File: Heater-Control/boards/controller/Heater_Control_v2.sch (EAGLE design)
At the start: 4 parts, among them J1 S2B-XH-A(LF)(SN), U1 QT Py #4600, X1 MLX-43860

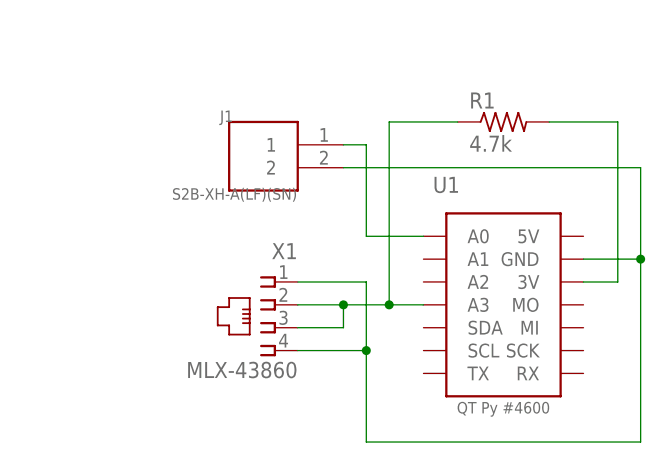
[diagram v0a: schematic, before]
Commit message: updated control board
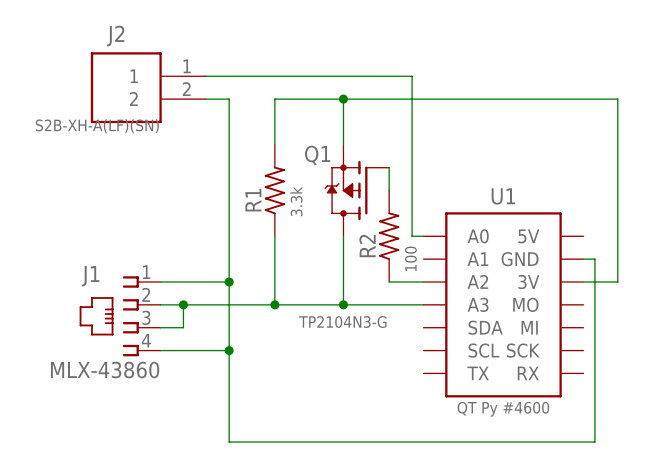
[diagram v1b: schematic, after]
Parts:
- removed X1: MLX-43860, home:MLX-43860
- added J2: S2B-XH-A(LF)(SN), Connectors:S2B-XH-A(LF)(SN)
- added Q1: TP2104N3-G, home:MOSFET-PCH-TO92
- added R2: 100, home:R-US_R1206
- J1: value S2B-XH-A(LF)(SN) -> MLX-43860; device Connectors:S2B-XH-A(LF)(SN) -> home:MLX-43860
- R1: value 4.7k -> 3.3k
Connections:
- new net GATE: Q1.G, R2.2
- new net SPU_GATE: R2.1, U1.A2
- net 3V3: now also Q1.S
- net DATA-1WIRE: now also J1.2, J1.3, Q1.D; no longer X1.2, X1.3
- net GND: now also J1.1, J1.4, J2.2; no longer J1.2, X1.1, X1.4
- net PWR: now also J2.1; no longer J1.1
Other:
- moved on the sheet: R1
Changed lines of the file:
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@@
 <setting verticaltext="up"/>
 </settings>
-<grid distance="0.1" unitdist="inch" unit="inch" style="lines" multiple="1" display="yes" altdistance="0.01" altunitdist="inch" altunit="inch"/>
+<grid distance="100" unitdist="mil" unit="mil" style="lines" multiple="1" display="yes" altdistance="50" altunitdist="mil" altunit="mil"/>
 <layers>
 <layer number="1" name="Top" color="4" fill="1" visible="no" active="no"/>
@@
 <class number="1" name="10mil" width="0.254" drill="0">
 </class>
+<class number="2" name="12mil" width="0.3048" drill="0">
+</class>
+<class number="3" name="8mil" width="0.2032" drill="0">
+</class>
 </classes>
 <parts>
 <part name="U1" library="home" deviceset="QT_PY" device="" value="QT Py #4600"/>
-<part name="X1" library="home" deviceset="MLX-43860" device=""/>
-<part name="J1" library="Connectors" library_urn="urn:adsk.eagle:library:14555660" deviceset="S2B-XH-A(LF)(SN)" device="" package3d_urn="urn:adsk.eagle:package:10989915/2"/>
-<part name="R1" library="home" deviceset="R-US_" device="R1206" package3d_urn="urn:adsk.eagle:package:23540/2" value="4.7k"/>
+<part name="J1" library="home" deviceset="MLX-43860" device=""/>
+<part name="J2" library="Connectors" library_urn="urn:adsk.eagle:library:14555660" deviceset="S2B-XH-A(LF)(SN)" device="" package3d_urn="urn:adsk.eagle:package:10989915/2"/>
+<part name="R1" library="home" deviceset="R-US_" device="R1206" package3d_urn="urn:adsk.eagle:package:23540/2" value="3.3k"/>
+<part name="Q1" library="home" deviceset="MOSFET-PCH" device="-TO92" value="TP2104N3-G"/>
+<part name="R2" library="home" deviceset="R-US_" device="R1206" package3d_urn="urn:adsk.eagle:package:23540/2" value="100"/>
 </parts>
 <sheets>
@@
 <instances>
 <instance part="U1" gate="G$1" x="38.1" y="15.24" smashed="yes">
-<attribute name="NAME" x="31.75" y="27.686" size="1.778" layer="95" ratio="10" align="bottom-center"/>
+<attribute name="NAME" x="38.1" y="26.416" size="1.778" layer="95" ratio="10" align="bottom-center"/>
 <attribute name="VALUE" x="38.1" y="4.445" size="1.27" layer="96" ratio="10" rot="R180" align="bottom-center"/>
 </instance>
-<instance part="X1" gate="G$1" x="12.7" y="12.7" smashed="yes" rot="MR0">
-<attribute name="NAME" x="15.24" y="20.32" size="1.778" layer="95" rot="MR0"/>
-<attribute name="VALUE" x="15.24" y="7.112" size="1.778" layer="96" rot="MR0"/>
-</instance>
-<instance part="J1" gate="G$1" x="10.16" y="30.48" smashed="yes">
-<attribute name="NAME" x="6.604" y="35.56" size="1.27" layer="95"/>
-<attribute name="VALUE" x="1.27" y="26.924" size="1.27" layer="96"/>
-</instance>
-<instance part="R1" gate="G$1" x="38.1" y="35.56" smashed="yes">
-<attribute name="NAME" x="34.29" y="37.0586" size="1.778" layer="95"/>
-<attribute name="VALUE" x="34.29" y="32.258" size="1.778" layer="96"/>
+<instance part="J1" gate="G$1" x="-2.54" y="12.7" smashed="yes" rot="MR0">
+<attribute name="NAME" x="-7.62" y="17.78" size="1.778" layer="95" ratio="10" rot="MR0" align="bottom-center"/>
+<attribute name="VALUE" x="0" y="7.112" size="1.778" layer="96" rot="MR0"/>
+</instance>
+<instance part="J2" gate="G$1" x="-5.08" y="38.1" smashed="yes">
+<attribute name="NAME" x="-4.826" y="44.45" size="1.778" layer="95" ratio="10" align="bottom-center"/>
+<attribute name="VALUE" x="-13.97" y="34.544" size="1.27" layer="96"/>
+</instance>
+<instance part="R1" gate="G$1" x="12.7" y="27.94" smashed="yes" rot="R90">
+<attribute name="NAME" x="11.2014" y="25.4" size="1.778" layer="95" ratio="10" rot="R90"/>
+<attribute name="VALUE" x="14.478" y="26.67" size="1.27" layer="96" ratio="10" rot="R270" align="bottom-center"/>
+</instance>
+<instance part="Q1" gate="G$1" x="20.32" y="27.94" smashed="yes" rot="MR0">
+<attribute name="VALUE" x="20.32" y="13.97" size="1.27" layer="96" rot="MR180" align="bottom-center"/>
+<attribute name="NAME" x="19.05" y="31.115" size="1.778" layer="95" ratio="10" rot="MR0"/>
+</instance>
+<instance part="R2" gate="G$1" x="25.4" y="22.86" smashed="yes" rot="R90">
+<attribute name="NAME" x="23.9014" y="20.32" size="1.778" layer="95" ratio="10" rot="R90"/>
+<attribute name="VALUE" x="27.178" y="20.32" size="1.27" layer="96" ratio="10" rot="R270" align="bottom-center"/>
 </instance>
 </instances>
@@
 </busses>
 <nets>
-<net name="GND" class="1">
+<net name="GND" class="2">
 <segment>
 <pinref part="U1" gate="G$1" pin="GND"/>
-<pinref part="X1" gate="G$1" pin="4"/>
-<wire x1="46.99" y1="20.32" x2="53.34" y2="20.32" width="0.1524" layer="91"/>
-<wire x1="15.24" y1="10.16" x2="22.86" y2="10.16" width="0.1524" layer="91"/>
-<wire x1="22.86" y1="10.16" x2="22.86" y2="0" width="0.1524" layer="91"/>
-<wire x1="22.86" y1="0" x2="53.34" y2="0" width="0.1524" layer="91"/>
-<wire x1="53.34" y1="0" x2="53.34" y2="20.32" width="0.1524" layer="91"/>
-<junction x="53.34" y="20.32"/>
-<pinref part="X1" gate="G$1" pin="1"/>
-<wire x1="15.24" y1="17.78" x2="22.86" y2="17.78" width="0.1524" layer="91"/>
-<wire x1="22.86" y1="17.78" x2="22.86" y2="10.16" width="0.1524" layer="91"/>
-<junction x="22.86" y="10.16"/>
-<wire x1="53.34" y1="30.48" x2="53.34" y2="20.32" width="0.1524" layer="91"/>
-<pinref part="J1" gate="G$1" pin="2"/>
-<wire x1="20.32" y1="30.48" x2="53.34" y2="30.48" width="0.1524" layer="91"/>
-</segment>
-</net>
-<net name="3V3" class="1">
+<pinref part="J1" gate="G$1" pin="4"/>
+<wire x1="46.99" y1="20.32" x2="48.26" y2="20.32" width="0.1524" layer="91"/>
+<wire x1="0" y1="10.16" x2="7.62" y2="10.16" width="0.1524" layer="91"/>
+<wire x1="7.62" y1="10.16" x2="7.62" y2="0" width="0.1524" layer="91"/>
+<wire x1="7.62" y1="0" x2="48.26" y2="0" width="0.1524" layer="91"/>
+<wire x1="48.26" y1="0" x2="48.26" y2="20.32" width="0.1524" layer="91"/>
+<pinref part="J1" gate="G$1" pin="1"/>
+<wire x1="0" y1="17.78" x2="7.62" y2="17.78" width="0.1524" layer="91"/>
+<wire x1="7.62" y1="17.78" x2="7.62" y2="10.16" width="0.1524" layer="91"/>
+<junction x="7.62" y="10.16"/>
+<pinref part="J2" gate="G$1" pin="2"/>
+<wire x1="5.08" y1="38.1" x2="7.62" y2="38.1" width="0.1524" layer="91"/>
+<wire x1="7.62" y1="17.78" x2="7.62" y2="38.1" width="0.1524" layer="91"/>
+<junction x="7.62" y="17.78"/>
+</segment>
+</net>
+<net name="3V3" class="2">
 <segment>
 <pinref part="U1" gate="G$1" pin="3V"/>
 <wire x1="46.99" y1="17.78" x2="50.8" y2="17.78" width="0.1524" layer="91"/>
 <pinref part="R1" gate="G$1" pin="2"/>
-<wire x1="50.8" y1="17.78" x2="50.8" y2="35.56" width="0.1524" layer="91"/>
-<wire x1="50.8" y1="35.56" x2="43.18" y2="35.56" width="0.1524" layer="91"/>
-</segment>
-</net>
-<net name="DATA-1WIRE" class="1">
-<segment>
-<pinref part="X1" gate="G$1" pin="2"/>
-<pinref part="X1" gate="G$1" pin="3"/>
-<wire x1="20.32" y1="15.24" x2="15.24" y2="15.24" width="0.1524" layer="91"/>
-<wire x1="15.24" y1="12.7" x2="20.32" y2="12.7" width="0.1524" layer="91"/>
-<wire x1="20.32" y1="12.7" x2="20.32" y2="15.24" width="0.1524" layer="91"/>
+<wire x1="50.8" y1="17.78" x2="50.8" y2="38.1" width="0.1524" layer="91"/>
+<wire x1="50.8" y1="38.1" x2="20.32" y2="38.1" width="0.1524" layer="91"/>
+<wire x1="12.7" y1="38.1" x2="12.7" y2="33.02" width="0.1524" layer="91"/>
+<wire x1="12.7" y1="38.1" x2="20.32" y2="38.1" width="0.1524" layer="91"/>
+<pinref part="Q1" gate="G$1" pin="S"/>
+<wire x1="20.32" y1="38.1" x2="20.32" y2="33.02" width="0.1524" layer="91"/>
+<junction x="20.32" y="38.1"/>
+</segment>
+</net>
+<net name="DATA-1WIRE" class="2">
+<segment>
+<pinref part="J1" gate="G$1" pin="2"/>
+<pinref part="J1" gate="G$1" pin="3"/>
+<wire x1="2.54" y1="15.24" x2="0" y2="15.24" width="0.1524" layer="91"/>
+<wire x1="0" y1="12.7" x2="2.54" y2="12.7" width="0.1524" layer="91"/>
+<wire x1="2.54" y1="12.7" x2="2.54" y2="15.24" width="0.1524" layer="91"/>
 <pinref part="U1" gate="G$1" pin="A3"/>
-<wire x1="29.21" y1="15.24" x2="25.4" y2="15.24" width="0.1524" layer="91"/>
+<wire x1="29.21" y1="15.24" x2="20.32" y2="15.24" width="0.1524" layer="91"/>
+<pinref part="R1" gate="G$1" pin="1"/>
+<wire x1="20.32" y1="15.24" x2="12.7" y2="15.24" width="0.1524" layer="91"/>
+<wire x1="12.7" y1="22.86" x2="12.7" y2="15.24" width="0.1524" layer="91"/>
+<junction x="12.7" y="15.24"/>
+<wire x1="2.54" y1="15.24" x2="12.7" y2="15.24" width="0.1524" layer="91"/>
+<junction x="2.54" y="15.24"/>
+<pinref part="Q1" gate="G$1" pin="D"/>
+<wire x1="20.32" y1="22.86" x2="20.32" y2="15.24" width="0.1524" layer="91"/>
 <junction x="20.32" y="15.24"/>
-<pinref part="R1" gate="G$1" pin="1"/>
-<wire x1="25.4" y1="15.24" x2="20.32" y2="15.24" width="0.1524" layer="91"/>
-<wire x1="33.02" y1="35.56" x2="25.4" y2="35.56" width="0.1524" layer="91"/>
-<wire x1="25.4" y1="35.56" x2="25.4" y2="15.24" width="0.1524" layer="91"/>
-<junction x="25.4" y="15.24"/>
 </segment>
 </net>
@@
 <segment>
 <pinref part="U1" gate="G$1" pin="A0"/>
-<wire x1="29.21" y1="22.86" x2="22.86" y2="22.86" width="0.1524" layer="91"/>
-<pinref part="J1" gate="G$1" pin="1"/>
-<wire x1="22.86" y1="22.86" x2="22.86" y2="33.02" width="0.1524" layer="91"/>
-<wire x1="22.86" y1="33.02" x2="20.32" y2="33.02" width="0.1524" layer="91"/>
-</segment>
-</net>
+<wire x1="29.21" y1="22.86" x2="27.94" y2="22.86" width="0.1524" layer="91"/>
+<pinref part="J2" gate="G$1" pin="1"/>
+<wire x1="27.94" y1="22.86" x2="27.94" y2="40.64" width="0.1524" layer="91"/>
+<wire x1="27.94" y1="40.64" x2="5.08" y2="40.64" width="0.1524" layer="91"/>
+</segment>
+</net>
+<net name="SPU_GATE" class="3">
+<segment>
+<pinref part="R2" gate="G$1" pin="1"/>
+<pinref part="U1" gate="G$1" pin="A2"/>
+<wire x1="25.4" y1="17.78" x2="29.21" y2="17.78" width="0.1524" layer="91"/>
+</segment>
+</net>
+<net name="GATE" class="3">
+<segment>
+<pinref part="R2" gate="G$1" pin="2"/>
+<pinref part="Q1" gate="G$1" pin="G"/>
+<wire x1="25.4" y1="27.94" x2="25.4" y2="30.48" width="0.1524" layer="91"/>
+</segment>
+</net>
